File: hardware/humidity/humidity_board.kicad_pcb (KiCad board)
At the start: 2 copper layers, 139 x 20 mm, 23 parts, among them IC1 ATMEGA88-A, J1 RJ45, P1 ISP, P2 UART, SW1 SW_RESET, U1 ST485, U2 HYT271, m3_loch VAL**

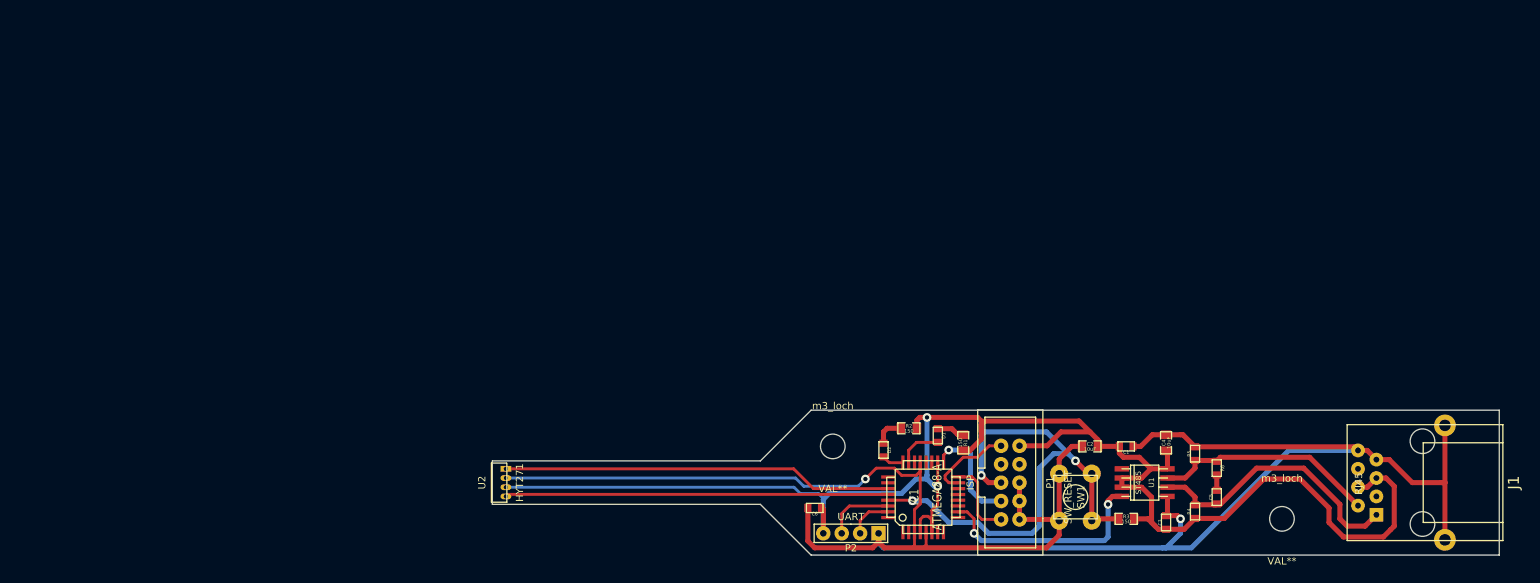
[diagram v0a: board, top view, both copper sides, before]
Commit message: checking
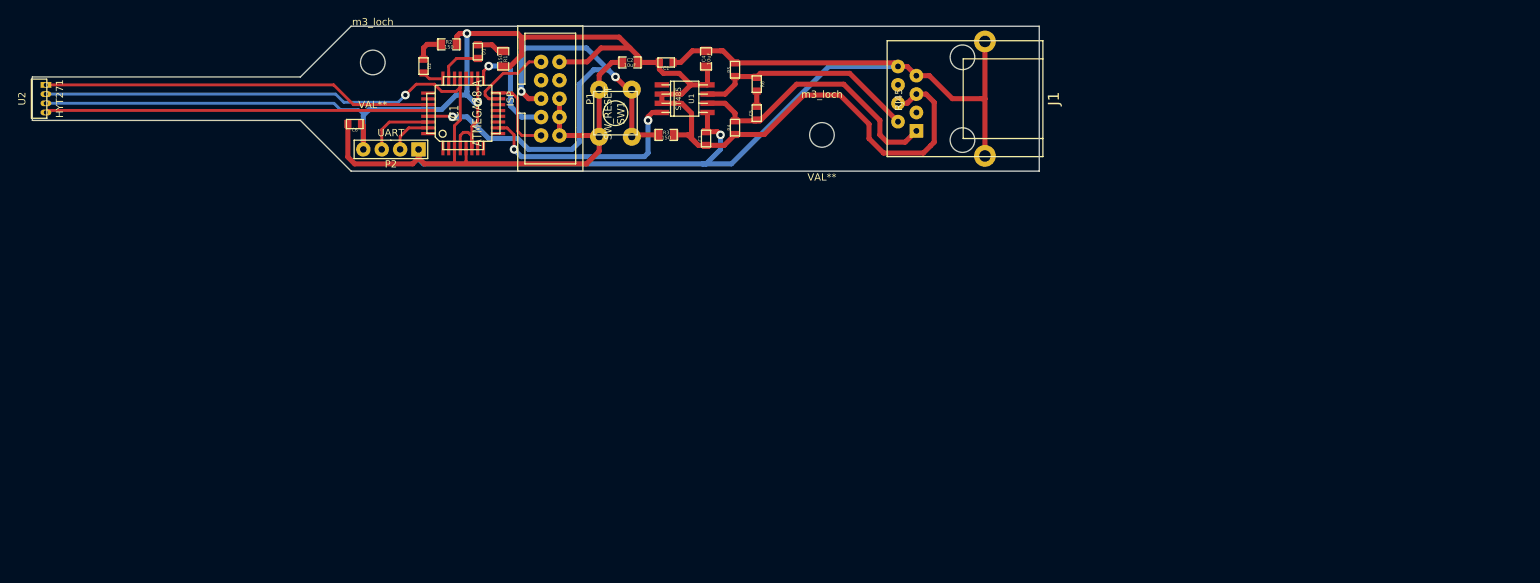
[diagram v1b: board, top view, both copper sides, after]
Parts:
- removed the m3_loch at (251.0, 154.0)
- removed the m3_loch at (189.0, 144.0)
- added m3_loch: VAL**, m3_loch, F.Cu at (187.5, 101.0)
- added m3_loch: VAL**, m3_loch, F.Cu at (125.5, 91.0)
- moved C1 82.7 mm to (166.0, 91.0)
- moved C2 82.7 mm to (161.0, 91.0)
- moved C3 82.7 mm to (171.5, 101.5)
- moved C4 82.7 mm to (171.5, 90.5)
- moved C5 82.7 mm to (178.5, 98.0)
- moved C6 82.7 mm to (123.0, 99.5)
- moved D1 82.7 mm to (140.0, 89.5)
- moved D2 82.7 mm to (132.5, 91.5)
- moved IC1 82.7 mm to (138.0, 98.0)
- moved J1 82.7 mm to (198.0, 96.0)
- moved P1 82.7 mm to (150.0, 96.0)
- moved P2 82.7 mm to (128.0, 103.0)
- moved R1 82.7 mm to (143.5, 90.5)
- moved R2 82.7 mm to (136.0, 88.5)
- moved R3 82.7 mm to (166.0, 101.0)
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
